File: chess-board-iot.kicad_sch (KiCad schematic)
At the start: 62 parts

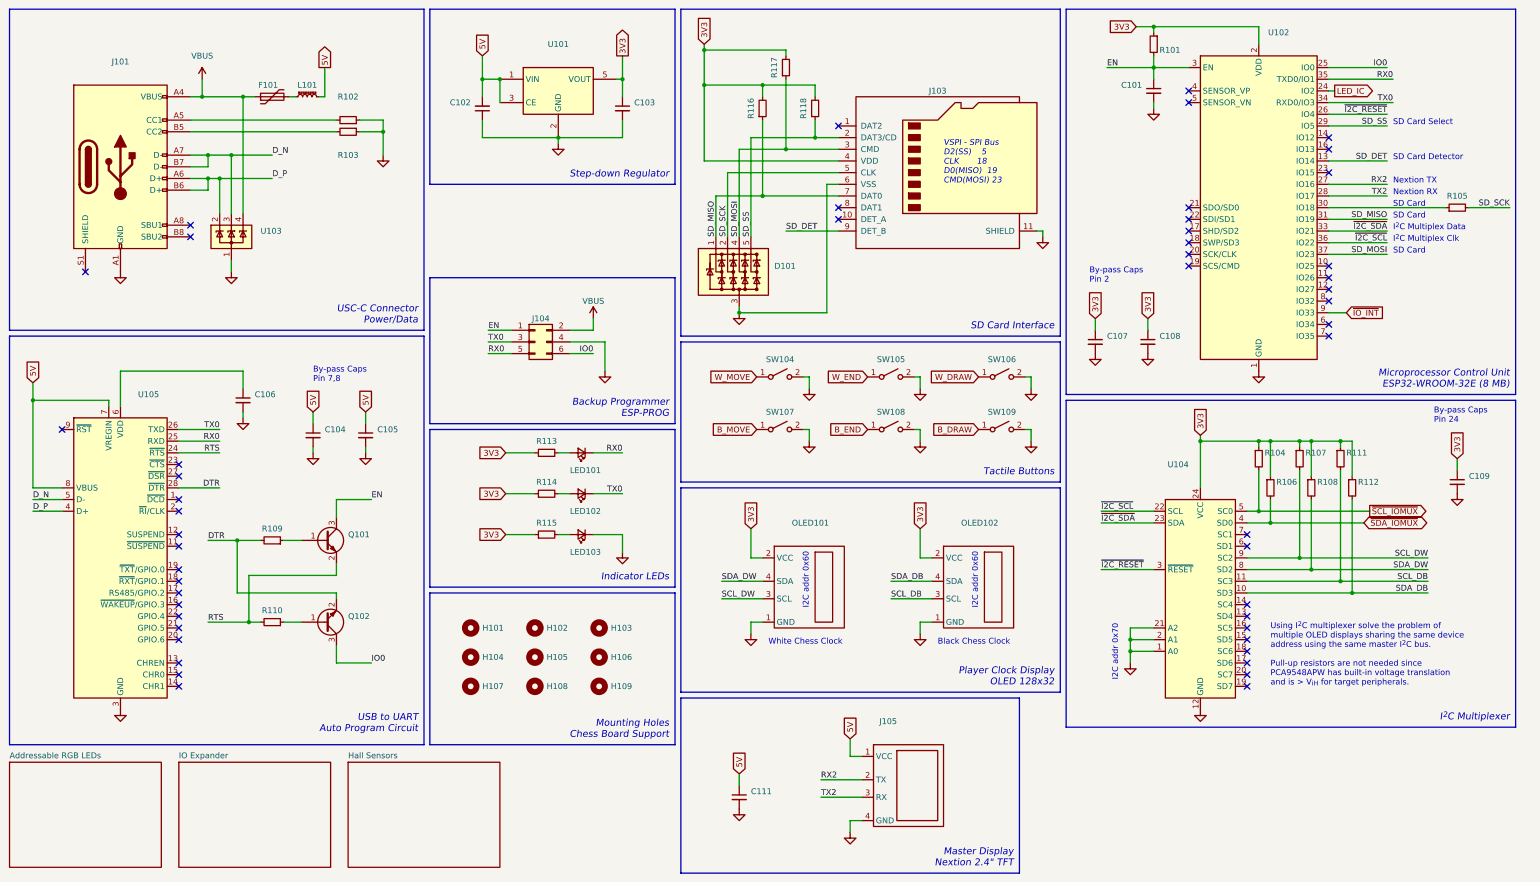
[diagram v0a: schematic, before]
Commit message: add pull ups, bypass caps for SD card
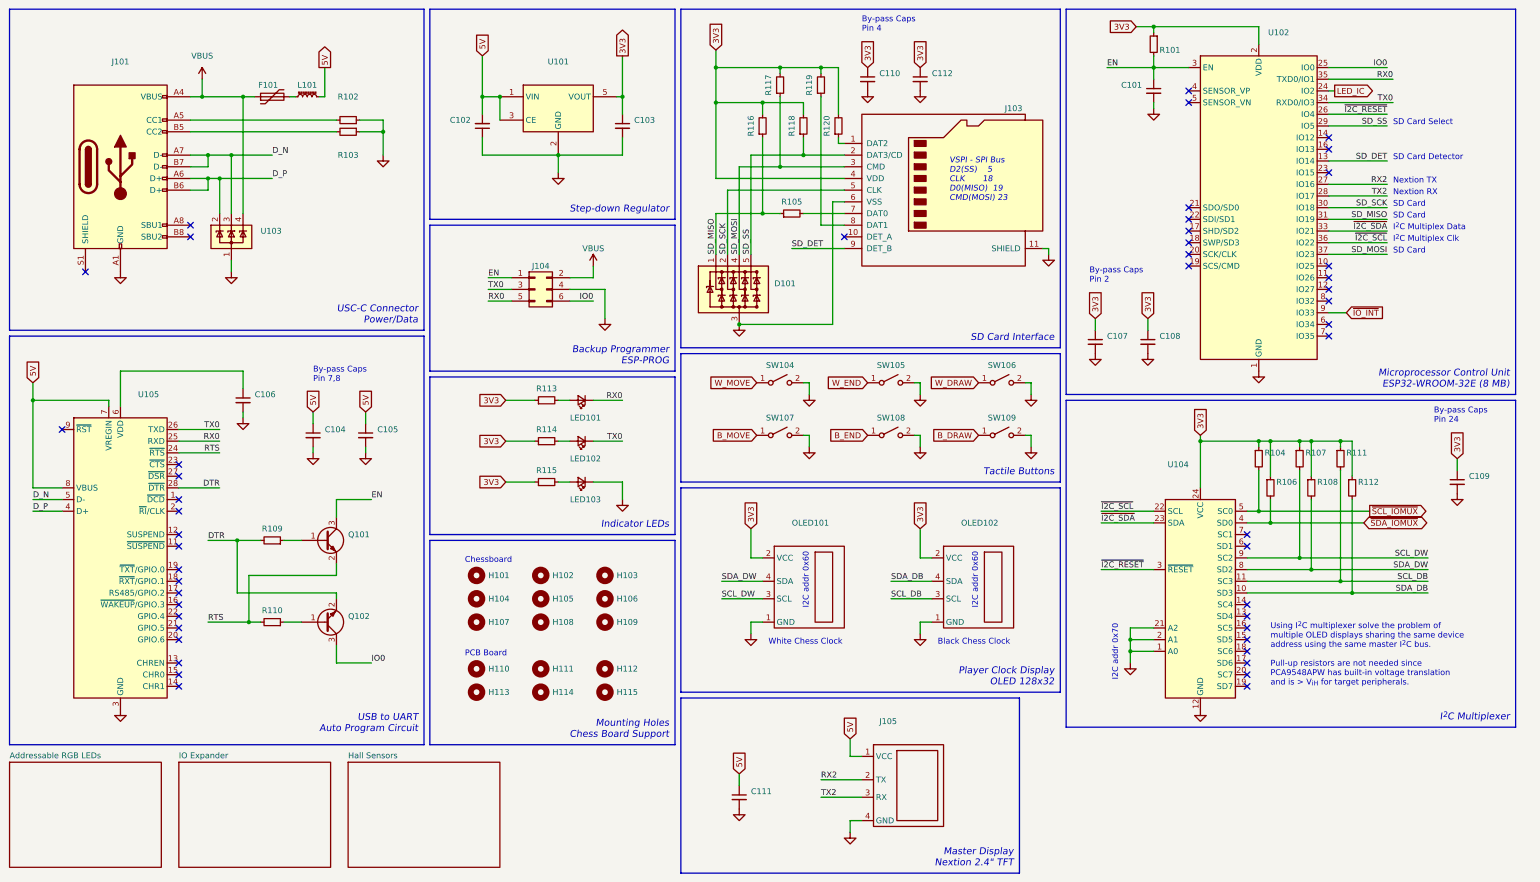
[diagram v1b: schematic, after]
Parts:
- added C110, C112: (no value), symbol Device:C_Small
- added H110, H111, H112, H113, H114, H115: (no value), symbol Mechanical:MountingHole
- added R119, R120: (no value), symbol Device:R_Small
- R116, R117, R118: LCSC C25804 -> C25819
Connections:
- net 3V3: now also C110.1, C112.1, R119.2, R120.2
- net GND: now also C110.2, C112.2
- net SD_MISO: now also R105.1; no longer J103.7 (DAT0)
- net SD_SCK: now also U102.30 (IO18); no longer R105.2
- net at J103.1 (DAT2): now also R120.1
- net at J103.8 (DAT1): now also R119.1
- new net: J103.7 (DAT0), R105.2
- no-connect marks 50 -> 48
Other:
- note added: "By-pass Caps Pin 4"
- note added: "Chessboard"
- note added: "PCB Board"
- moved on the sheet: C102, C103, D101, H101, H102, H103, H104, H105, H106, H107, H108, H109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
